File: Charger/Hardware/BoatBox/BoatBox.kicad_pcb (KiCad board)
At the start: 2 copper layers, 119 parts, among them P101 TestPoint, P102 TestPoint, P103 TestPoint, P104 TestPoint, P105 TestPoint, P106 TestPoint, P107 TestPoint, P108 TestPoint, P109 TestPoint, P110 TestPoint, P111 TestPoint, P112 TestPoint, P113 TestPoint, P114 TestPoint, P115 TestPoint, P116 TestPoint, P117 TestPoint, P118 TestPoint, P119 TestPoint, P120 TestPoint, P201 TestPoint, P202 TestPoint, P301 TestPoint, P302 TestPoint, P401 TestPoint, P402 TestPoint, P501 TestPoint, P502 TestPoint, T101 IRFR5505PBF, T102 BSS138, T103 IRFR5505PBF, T201 BC847, T202 IPD50R380CE, T203 BSS138, T301 BC847, T302 IPD50R380CE, T303 BSS138, T401 BC847, T402 IPD50R380CE, T403 BSS138, T501 BC847, T502 IPD50R380CE, T503 BSS138, X101 HCCPHPE24BKA90F

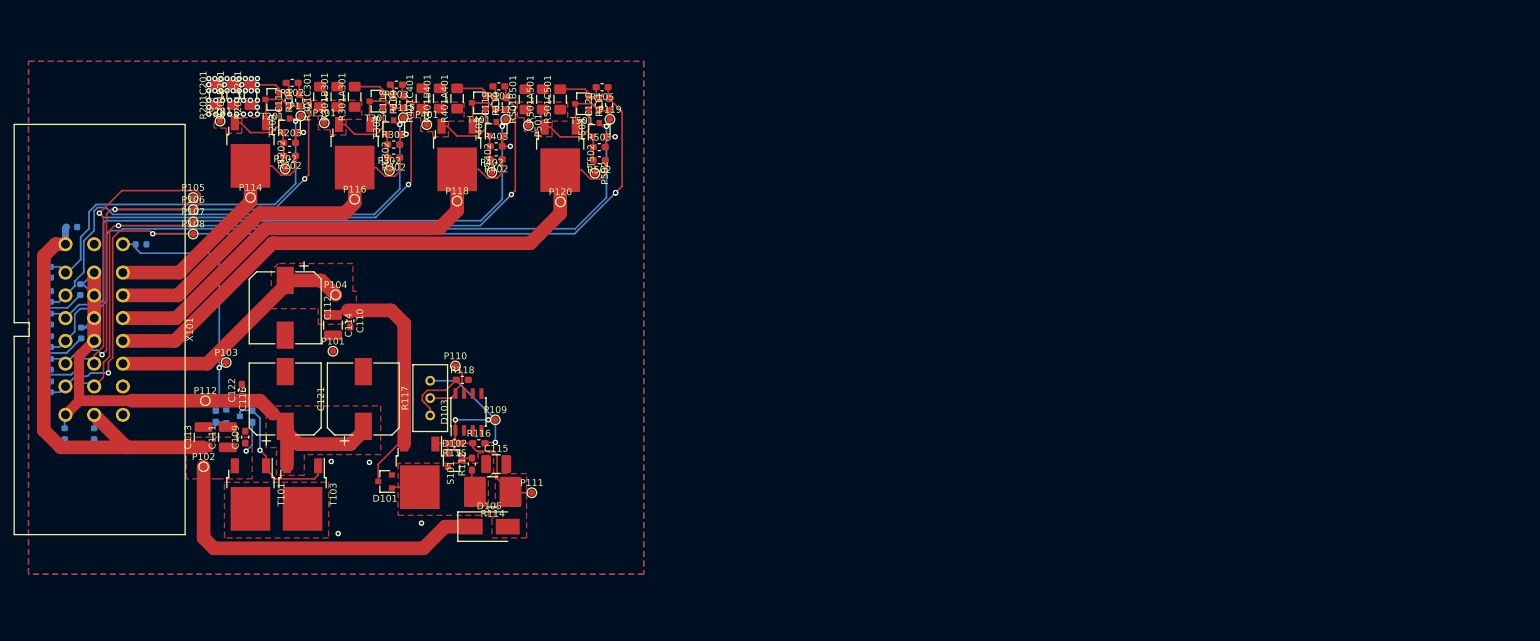
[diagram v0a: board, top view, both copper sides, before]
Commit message: WIP commit
squash after finish.
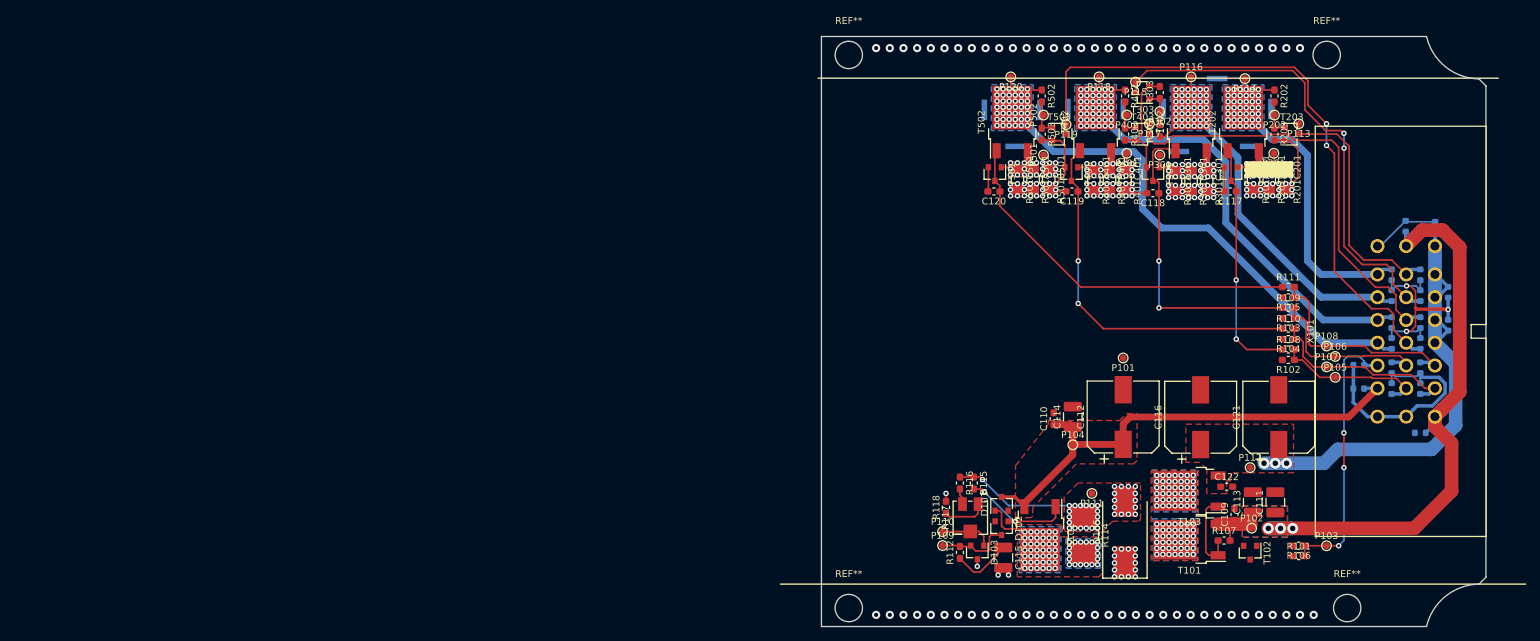
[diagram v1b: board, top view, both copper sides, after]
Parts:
- added ?: , boatbox:Zeichnung, F.Cu at (293.4, 149.0)
- added REF**: MountingHole_4mm, MountingHole:MountingHole_4mm, F.Cu at (237.9, 150.0)
- added REF**: BUMP-SR0.8-3.0, boatbox:BUMP-SR0.8-3.0, B.Cu at (218.9, 72.5)
- added REF**: BUMP-SR0.8-3.0, boatbox:BUMP-SR0.8-3.0, B.Cu at (211.0, 77.0)
- added REF**: BUMP-SR0.8-3.0, boatbox:BUMP-SR0.8-3.0, B.Cu at (205.1, 77.0)
- added REF**: BUMP-SR0.8-3.0, boatbox:BUMP-SR0.8-3.0, B.Cu at (197.0, 77.0)
- added REF**: BUMP-SR0.8-3.0, boatbox:BUMP-SR0.8-3.0, B.Cu at (184.8, 77.1)
- added REF**: MountingHole_4mm, MountingHole:MountingHole_4mm, F.Cu at (234.9, 69.1)
- added REF**: MountingHole_4mm, MountingHole:MountingHole_4mm, F.Cu at (165.0, 69.1)
- added REF**: MountingHole_4mm, MountingHole:MountingHole_4mm, F.Cu at (165.0, 150.0)
- added REF**: BUMP-SR0.8-3.0, boatbox:BUMP-SR0.8-3.0, B.Cu at (223.7, 82.4)
- added REF**: BUMP-SR0.8-3.0, boatbox:BUMP-SR0.8-3.0, B.Cu at (213.3, 83.2)
- added REF**: BUMP-SR0.8-3.0, boatbox:BUMP-SR0.8-3.0, B.Cu at (189.4, 82.4)
- added REF**: BUMP-SR0.8-3.0, boatbox:BUMP-SR0.8-3.0, B.Cu at (192.9, 77.1)
- added REF**: BUMP-SR0.8-3.0, boatbox:BUMP-SR0.8-3.0, B.Cu at (226.7, 77.0)
- D103: value TL431D -> NCP431; footprint Package_SO:SOIC-8_3.9x4.9mm_P1.27mm -> Package_TO_SOT_SMD:SOT-23
- D105: footprint Diode_SMD:D_SMB_Handsoldering -> Diode_SMD:D_SMC_Handsoldering
- R101, R106, R107, T102: moved to F.Cu
- R117: footprint Potentiometer_THT:Potentiometer_Bourns_3296W_Vertical -> boatbox:Potentiometer_Cemet_23A_Horizontal
- moved C124 202.7 mm to (250.8, 94.3), turned to 270 degrees
- moved C108 200.3 mm to (248.6, 114.8), turned to 90 degrees
- moved C133 200.3 mm to (248.6, 108.2)
- moved C127 200.3 mm to (248.6, 101.2)
- moved C131 200.3 mm to (248.6, 111.3)
- moved C129 200.3 mm to (248.6, 104.3)
- moved C125 200.1 mm to (252.6, 108.6), turned to 270 degrees
- moved C126 200.0 mm to (252.6, 103.8)
- moved C101 199.5 mm to (248.6, 124.3), turned to 0 degrees
- moved C105 196.2 mm to (244.4, 117.9), turned to 270 degrees
- moved C107 196.0 mm to (248.6, 117.9), turned to 270 degrees
- moved C102 194.2 mm to (246.4, 94.1), turned to 270 degrees
- moved X101 191.9 mm to (246.5, 109.5), turned to 90 degrees
- moved C106 191.8 mm to (244.4, 114.8)
- moved C134 182.9 mm to (244.4, 108.2), turned to 90 degrees
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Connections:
- D103 pad 1: Net-(D102-Pad1) -> Net-(D103-Pad1)
- D103 pad 2: GND -> Net-(D102-Pad1)
- P110 pad 1: Net-(D103-Pad8) -> Net-(D103-Pad1)
- R117 pad 2: Net-(D103-Pad8) -> Net-(D103-Pad1)
- X101 pad 10: UBR -> /E_S_CTL1
- X101 pad 11: UBR -> /E_S_CTL2
- X101 pad 12: UBR -> /A_S_DIAG4
- X101 pad 13: UBR -> /A_S_DIAG3
- X101 pad 14: /E_S_CTL2 -> /A_S_DIAG2
- X101 pad 15: /E_S_CTL3 -> /A_S_DIAG1
- X101 pad 17: /E_S_RLY -> GND
- X101 pad 18: /A_T_OUT1 -> /U_U_CHRG
- X101 pad 19: /A_T_OUT2 -> /E_S_RLY
- X101 pad 2: /A_S_DIAG1 -> /E_S_CTL3
- X101 pad 20: /A_T_OUT3 -> /A_T_OUT4
- X101 pad 21: /A_T_OUT4 -> /A_T_OUT3
- X101 pad 22: /U_U_CHRG -> /A_T_OUT2
- X101 pad 23: GND -> /A_T_OUT1
- X101 pad 3: /A_S_DIAG2 -> /E_S_CTL4
- X101 pad 4: /A_S_DIAG3 -> UBR
- X101 pad 5: /A_S_DIAG4 -> UBR
- X101 pad 6: /E_S_CTL1 -> UBR
- X101 pad 7: /E_S_CTL4 -> UBR
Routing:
- net /E_S_CTL4: track 128.8 -> 32.2 mm, vias 4 -> 0
- net /E_S_CTL3: track 114.8 -> 28.8 mm, vias 2 -> 0
- net /E_S_CTL2: track 106.9 -> 26.0 mm, vias 2 -> 0
- net GND: track 64.8 -> 133.3 mm, vias 30 -> 152
- net /E_S_CTL1: track 87.9 -> 22.1 mm, vias 3 -> 0
- net /LSS 3/ctrl: track 8.82 -> 54.7 mm, vias 0 -> 2
- net /LSS 4/ctrl: track 8.86 -> 54.7 mm
- net /LSS 2/ctrl: track 8.82 -> 45.4 mm, vias 0 -> 2
- net /A_S_DIAG3: track 93.1 -> 64.2 mm, vias 1 -> 0
- net UBD: track 121.1 -> 93.7 mm, vias 1 -> 17
- net /LSS 1/ctrl: track 8.82 -> 35.8 mm, vias 0 -> 2
- net /A_S_DIAG1: track 56.2 -> 36.6 mm, vias 1 -> 0
- net /A_S_DIAG4: track 110.5 -> 93.7 mm, vias 1 -> 2
- net Net-(R116-Pad2): track 16.8 -> 2.36 mm, vias 1 -> 0
- net UBR: track 84.7 -> 70.3 mm, vias 0 -> 3
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- added copper zone on B.Cu, net /A_T_OUT1
- added copper zone on B.Cu, net /A_T_OUT2
- added copper zone on B.Cu, net /A_T_OUT3
- added copper zone on B.Cu, net /A_T_OUT4
- added copper zone on B.Cu, net Net-(C115-Pad1)
- added copper zone on B.Cu, net Net-(P201-Pad1)
- added copper zone on B.Cu, net Net-(P301-Pad1)
- added copper zone on B.Cu, net Net-(P401-Pad1)
- added copper zone on B.Cu, net Net-(P501-Pad1)
- added copper zone on B.Cu, net Net-(T101-Pad2)
- added copper zone on B.Cu, net UBD
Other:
- board outline added: 97.2 x 86.3 mm
- net class 3A added: clearance 0.3, trace_width 1, via_dia 1.6, via_drill 0.8
- net class 6A added: clearance 0.3, trace_width 2, via_dia 1.6, via_drill 0.8
